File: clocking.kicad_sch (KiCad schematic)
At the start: 41 parts

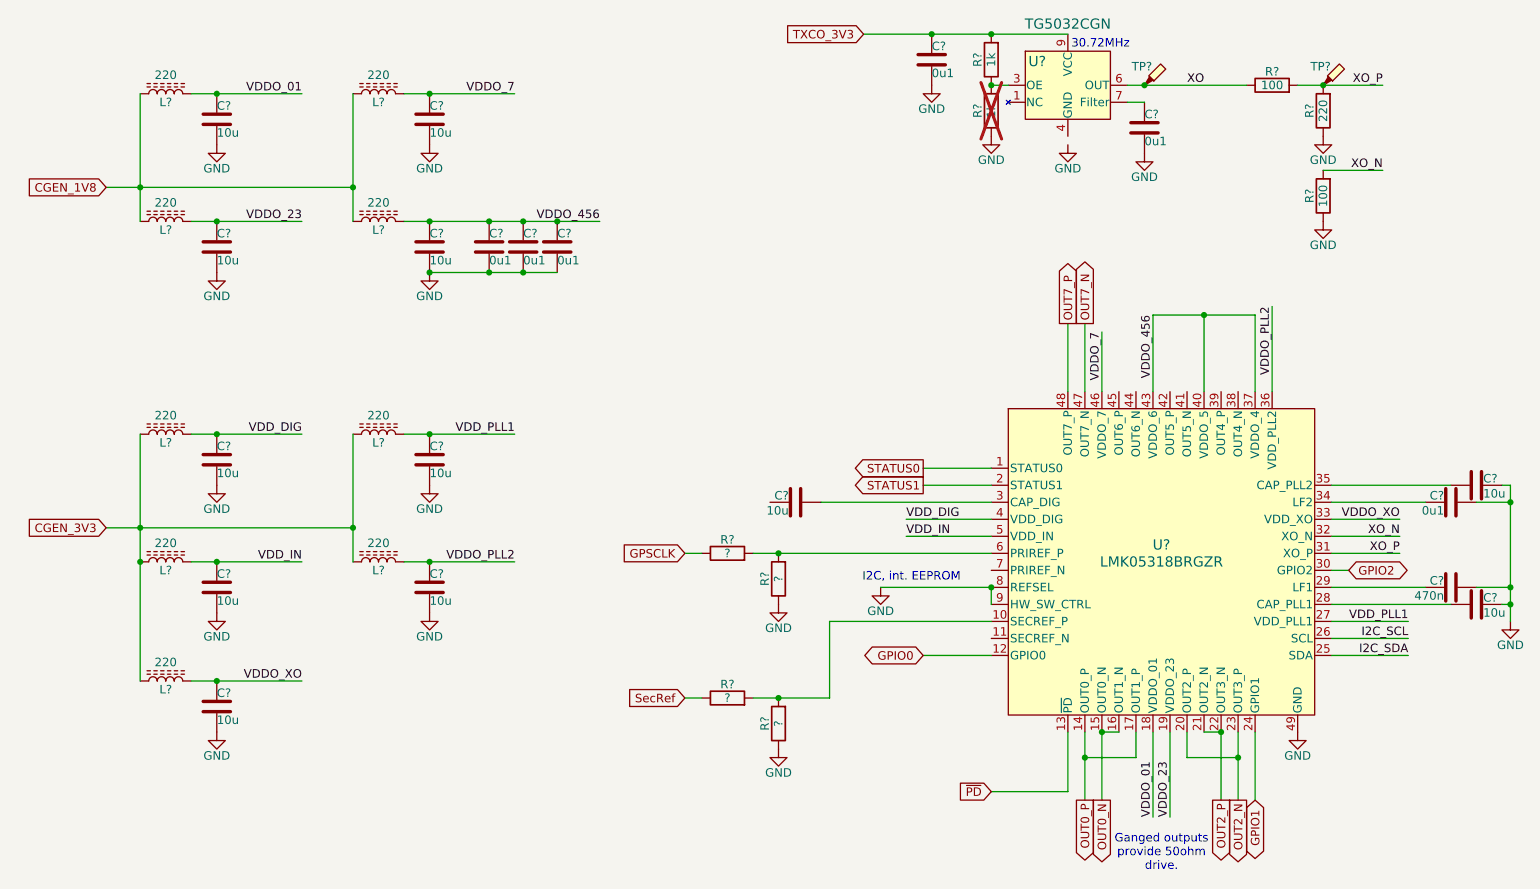
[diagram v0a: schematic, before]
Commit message: Schematic is basically feature complete
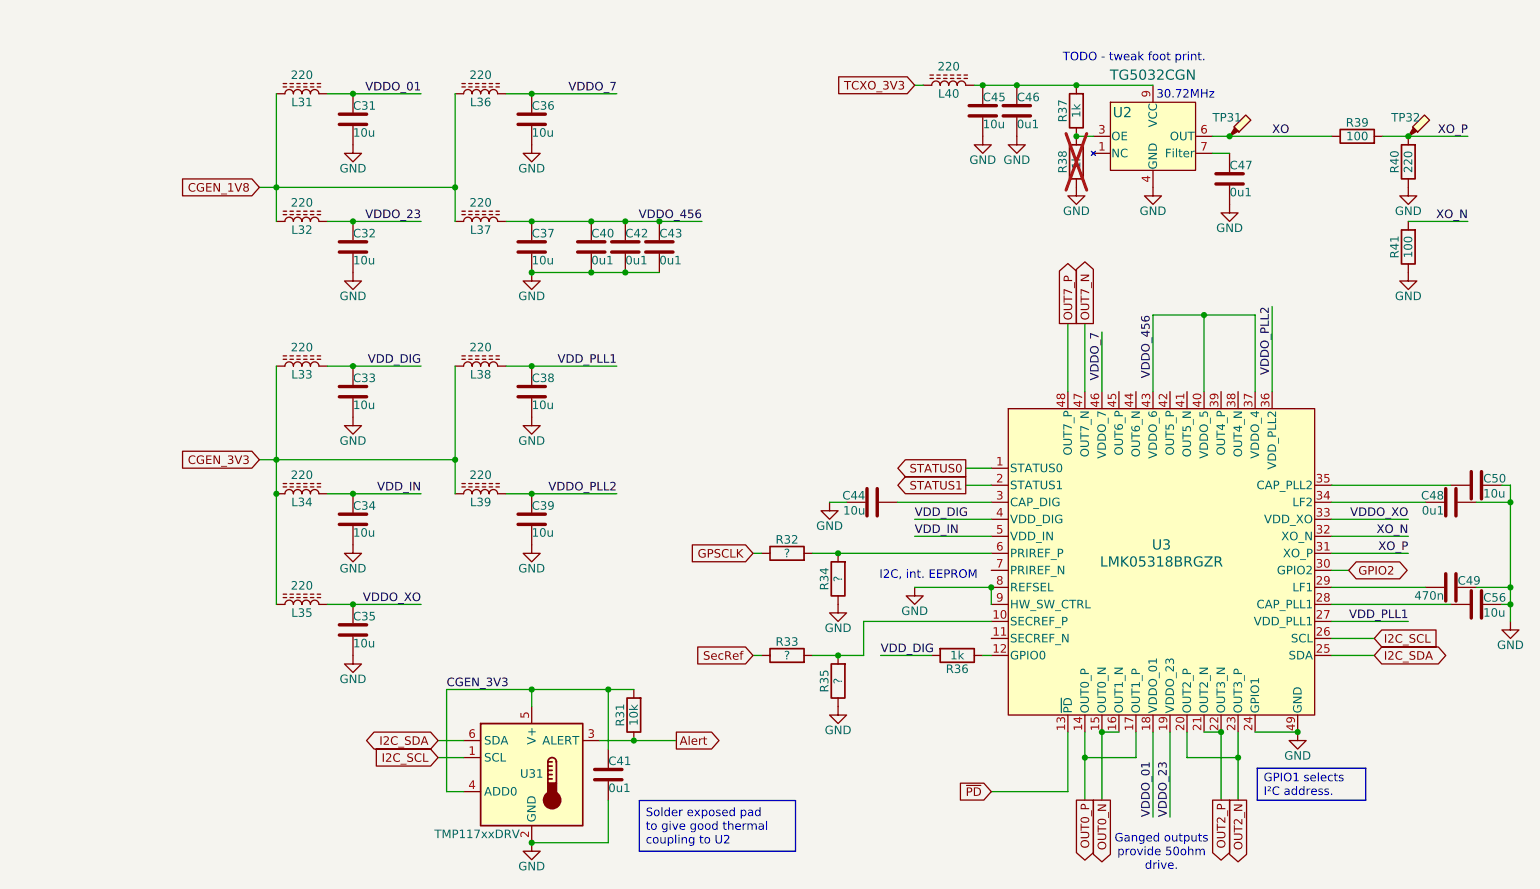
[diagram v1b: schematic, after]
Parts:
- added C41: 0u1, Capacitor_SMD:C_0402_1005Metric, symbol Device:C
- added C45: 10u, Capacitor_SMD:C_0402_1005Metric, symbol Device:C
- added L40: 220, Inductor_SMD:L_0603_1608Metric, symbol Device:L_Ferrite
- added R31: 10k, symbol Device:R
- added R36: 1k, Resistor_SMD:R_0603_1608Metric, symbol Device:R
- added U31: TMP117xxDRV, Package_SON:WSON-6-1EP_2x2mm_P0.65mm_NoEP, symbol Parts:TMP117xxDRV
- C31, C32, C33, C34, C35, C36, C37, C38, C39, C44, C50, C56: renamed from C?; JLCPCB (none) -> C15525
- L31, L32, L33, L34, L35, L36, L37, L38, L39: renamed from L?; footprint (none) -> Inductor_SMD:L_0603_1608Metric; JLCPCB (none) -> C14709
- R40: renamed from R?; footprint (none) -> Inductor_SMD:L_0603_1608Metric; JLCPCB (none) -> C14709
- R41: renamed from R?; footprint 0603? -> (none)
- TP31, TP32: renamed from TP?; now left out of the parts list
- U2: renamed from U?; JLCPCB (none) -> C2891970
- U3: renamed from U?; JLCPCB (none) -> C3611586
- gave numbers to parts that had none: 14
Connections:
- net GPIO1 is gone; now on net GND: U3.24 (GPIO1)
- net CGEN_3V3: now also C41.1, R31.2, U31.4 (ADD0), U31.5 (V+)
- net GND: now also C44.1, U2.4 (GND), C41.2, C45.2, U31.2 (GND)
- net I2C_SCL: now also U31.1 (SCL)
- net I2C_SDA: now also U31.6 (SDA)
- net VDD_DIG: now also R36.2
- net GPIO0: no longer names the net of U3.12 (GPIO0)
- net GPIO0: now also R36.1
- net TXCO_3V3: no longer names the net of C46.1, R37.2, U2.9 (VCC)
- net TXCO_3V3: now also C45.1, L40.2
- new net Alert: R31.1, U31.3 (ALERT)
- new net TCXO_3V3: L40.1
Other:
- note added: "TODO - tweak foot print."
- moved on the sheet: C31, C32, C33, C34, C35, C36, C37, C38, C39, C40, C42, C43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
